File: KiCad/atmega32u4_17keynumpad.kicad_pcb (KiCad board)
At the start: 2 copper layers, 82 x 134 mm, 50 parts, among them SW1 1825115-1, SW10 MX1A-11NW, SW11 MX1A-11NW, SW118 MX1A-11NW, SW12 MX1A-11NW, SW13 MX1A-11NW, SW14 MX1A-11NW, SW15 MX1A-11NW, SW16 MX1A-11NW, SW17 MX1A-11NW, SW2 MX1A-11NW, SW3 MX1A-11NW, SW4 MX1A-11NW, SW5 MX1A-11NW, SW6 MX1A-11NW, SW7 MX1A-11NW, SW8 MX1A-11NW, SW9 MX1A-11NW

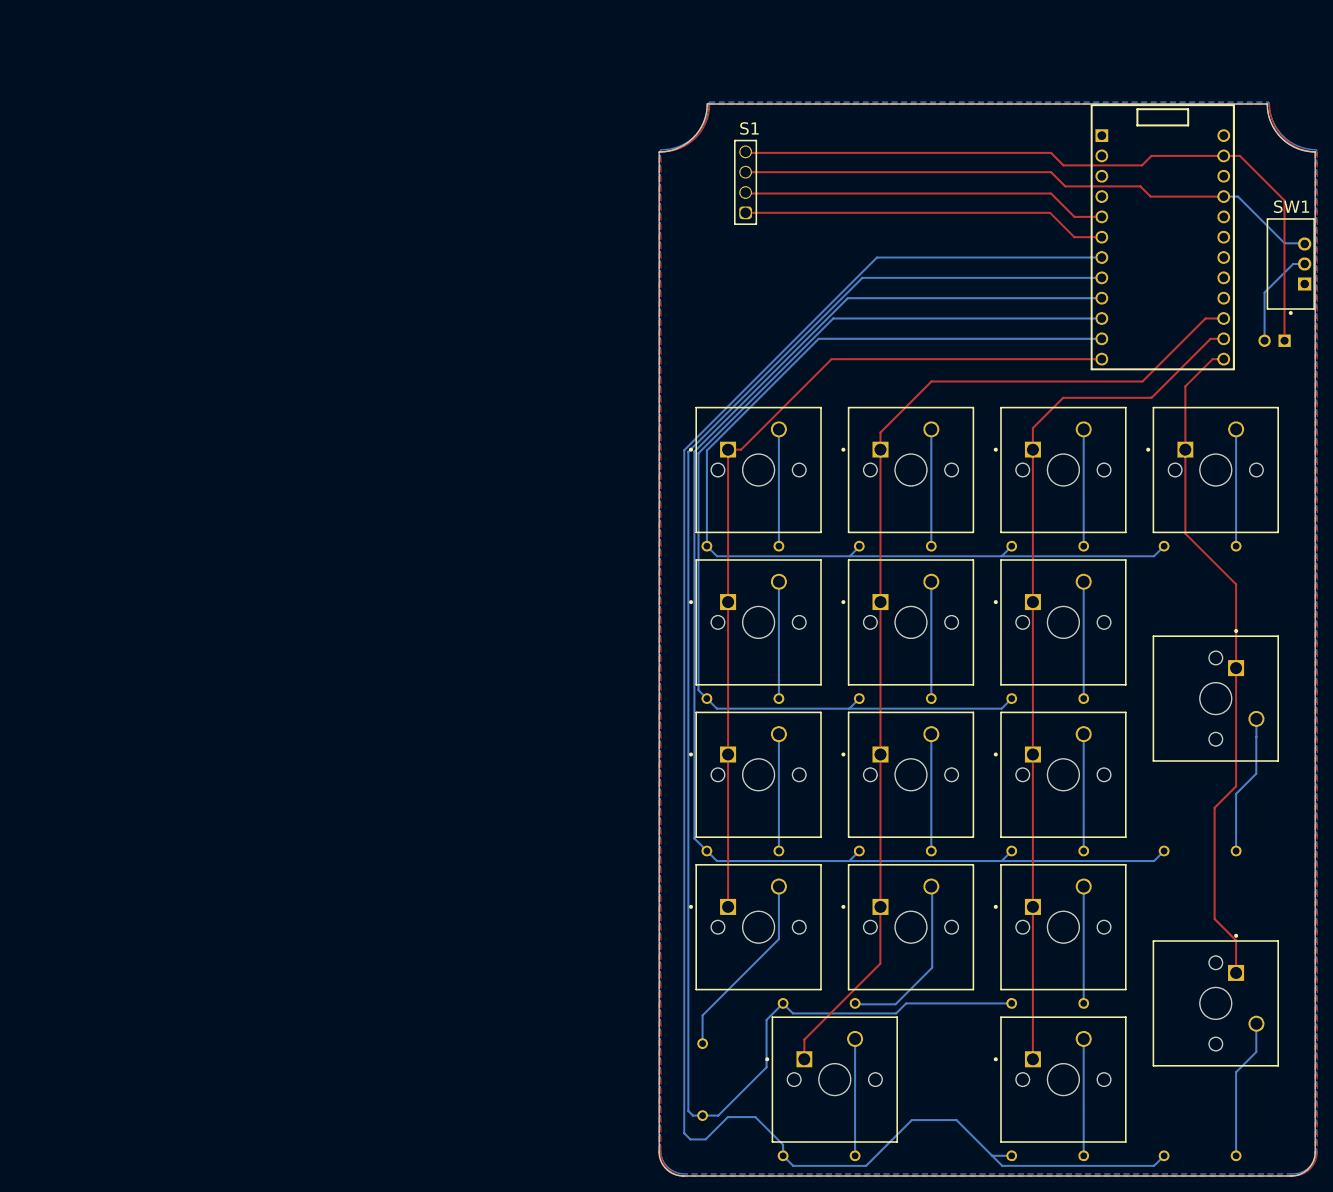
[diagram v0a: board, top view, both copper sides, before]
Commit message: finished pcb
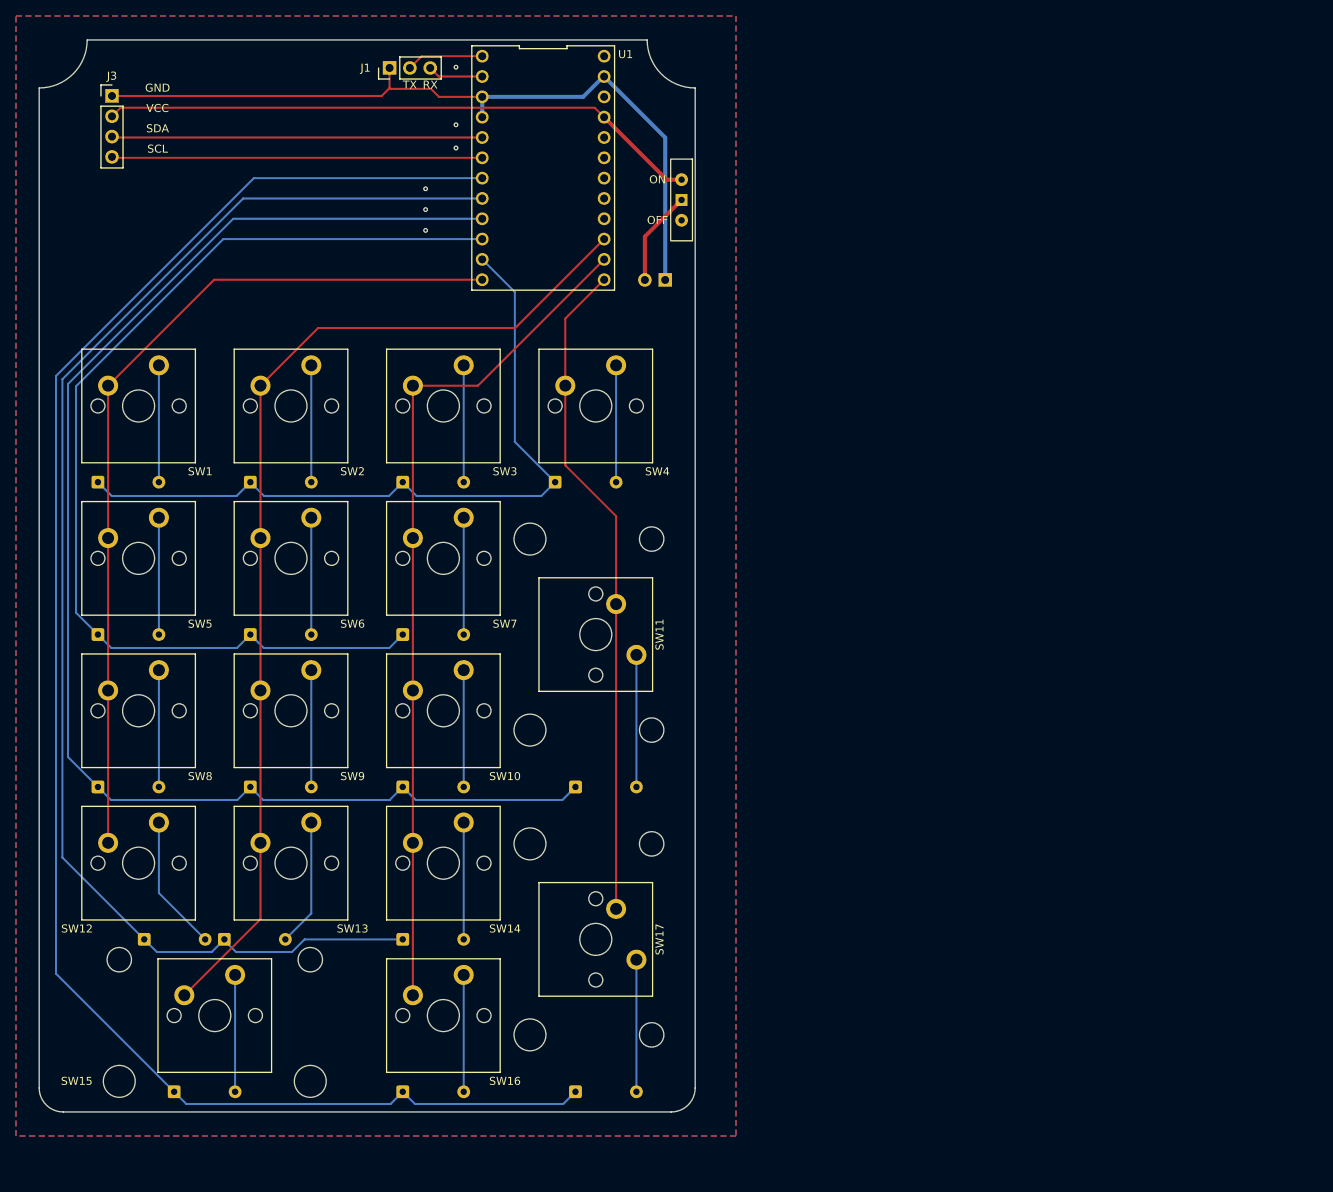
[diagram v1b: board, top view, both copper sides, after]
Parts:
- removed ? (x12): , 
- removed ?: PRO MICRO, PcbLib1:PRO MICRO
- removed B1: B2B-XH-A(LF)(SN), Vault:FP-B2B-XH-A_LF_SN-MFG
- removed D18: 1N4148, Vault:NXP-SOD27-2_V
- removed S1: 61300411121, Vault:61300411121
- removed SW118: MX1A-11NW, Vault:CHRY-MX1A-11NW_V
- added D1: 1N4148, Diode_THT:D_DO-35_SOD27_P7.62mm_Horizontal, B.Cu at (37.3, 85.3)
- added J1: Conn_01x03_Pin, Connector_PinHeader_2.54mm:PinHeader_1x03_P2.54mm_Vertical, F.Cu at (73.8, 33.5)
- added J2: power supply, Connector_PinSocket_2.54mm:PinSocket_1x02_P2.54mm_Vertical, B.Cu at (108.2, 60.0)
- added J3: LCD1602, Connector_PinHeader_2.54mm:PinHeader_1x04_P2.54mm_Vertical, F.Cu at (39.1, 37.0)
- added REF**: Stabilizer_Cherry_MX_2.00u, PCM_Mounting_Keyboard_Stabilizer:Stabilizer_Cherry_MX_2.00u, F.Cu at (99.6, 104.3)
- added REF**: Stabilizer_Cherry_MX_2.00u, PCM_Mounting_Keyboard_Stabilizer:Stabilizer_Cherry_MX_2.00u, F.Cu at (52.0, 151.9)
- added REF**: Stabilizer_Cherry_MX_2.00u, PCM_Mounting_Keyboard_Stabilizer:Stabilizer_Cherry_MX_2.00u, F.Cu at (99.6, 142.4)
- added SW18: slide_switch, Button_Switch_THT:SW_Slide-03_Wuerth-WS-SLTV_10x2.5x6.4_P2.54mm, F.Cu at (110.3, 50.0)
- added U1: Pro Micro, pro_micro:Pro Micro, F.Cu at (93.0, 46.0)
- D10, D11, D12, D13, D14, D15, D16, D17, D2, D3, D4, D5, D6, D7, D8, D9: footprint Vault:NXP-SOD27-2_V -> Diode_THT:D_DO-35_SOD27_P7.62mm_Horizontal
- SW1: value 1825115-1 -> SW_Push; footprint Vault:FP-1825115-1-MFG -> PCM_Switch_Keyboard_Cherry_MX:SW_Cherry_MX_PCB_1.00u
- SW10, SW12, SW13, SW14, SW16, SW2, SW3, SW4, SW5, SW6, SW7, SW8, SW9: value MX1A-11NW -> SW_Push; footprint Vault:CHRY-MX1A-11NW_V -> PCM_Switch_Keyboard_Cherry_MX:SW_Cherry_MX_PCB_1.00u
- SW11, SW15, SW17: value MX1A-11NW -> SW_Push; footprint Vault:CHRY-MX1A-11NW_V -> PCM_Switch_Keyboard_Cherry_MX:SW_Cherry_MX_PCB_2.00u
- moved SW1 145.1 mm to (42.4, 75.8), turned to 0 degrees
- moved D5 138.2 mm to (37.3, 104.3), turned to 0 degrees
- moved SW12 136.2 mm to (42.4, 132.9), turned to 0 degrees
- moved SW5 135.1 mm to (42.4, 94.8)
- moved D12 132.4 mm to (43.1, 142.4), turned to 0 degrees
- moved D8 119.2 mm to (37.3, 123.4), turned to 0 degrees
- moved SW8 116.1 mm to (42.4, 113.8)
- moved D15 109.8 mm to (46.9, 161.5), turned to 0 degrees
- moved SW15 106.6 mm to (52.0, 151.9)
- moved D13 62.3 mm to (53.1, 142.4), turned to 0 degrees
- moved D10 62.1 mm to (75.4, 123.4), turned to 0 degrees
- moved D3 62.1 mm to (75.4, 85.3), turned to 0 degrees
- moved D4 62.1 mm to (94.5, 85.3), turned to 0 degrees
- moved D7 62.1 mm to (75.4, 104.3), turned to 0 degrees
- moved D2 62.1 mm to (56.4, 85.3), turned to 0 degrees
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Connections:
- net NetMCU1_15 renamed /Pin 16 (COL 3)
- D10 pad 1: NetD10_1 -> /Pin 6 (ROW 3)
- D10 pad 2: NetD9_2 -> Net-(D10-A)
- D11 pad 1: NetD11_1 -> /Pin 6 (ROW 3)
- D11 pad 2: NetD9_2 -> Net-(D11-A)
- D12 pad 1: NetD12_1 -> /Pin 5 (ROW 4)
- D12 pad 2: NetD9_2 -> Net-(D12-A)
- D13 pad 1: NetD13_1 -> /Pin 5 (ROW 4)
- D13 pad 2: NetD13_2 -> Net-(D13-A)
- D14 pad 1: NetD14_1 -> /Pin 5 (ROW 4)
- D14 pad 2: NetD13_2 -> Net-(D14-A)
- D15 pad 1: NetD15_1 -> /Pin 4 (ROW 5)
- D15 pad 2: NetD13_2 -> Net-(D15-A)
- D16 pad 1: NetD16_1 -> /Pin 4 (ROW 5)
- D16 pad 2: NetD16_2 -> Net-(D16-A)
- D17 pad 1: NetD17_1 -> /Pin 4 (ROW 5)
- D17 pad 2: NetD16_2 -> Net-(D17-A)
- D2 pad 1: NetD2_1 -> /Pin 8 (ROW 1)
- D2 pad 2: NetD2_2 -> Net-(D2-A)
- D3 pad 1: NetD3_1 -> /Pin 8 (ROW 1)
- D3 pad 2: NetD2_2 -> Net-(D3-A)
- D4 pad 1: NetD4_1 -> /Pin 8 (ROW 1)
- D4 pad 2: NetD2_2 -> Net-(D4-A)
- D5 pad 1: NetD5_1 -> /Pin 7 (ROW 2)
- D5 pad 2: NetD2_2 -> Net-(D5-A)
- D6 pad 1: NetD6_1 -> /Pin 7 (ROW 2)
- D6 pad 2: NetD6_2 -> Net-(D6-A)
- D7 pad 1: NetD7_1 -> /Pin 7 (ROW 2)
- D7 pad 2: NetD6_2 -> Net-(D7-A)
- D8 pad 1: NetD8_1 -> /Pin 6 (ROW 3)
- D8 pad 2: NetD6_2 -> Net-(D8-A)
- D9 pad 1: NetD9_1 -> /Pin 6 (ROW 3)
- D9 pad 2: NetD9_2 -> Net-(D9-A)
- SW1 pad 1: (no net) -> /Pin 9 (COL 1)
- SW1 pad 2: NetJ1_2 -> Net-(D1-A)
- SW10 pad 2: NetD10_1 -> Net-(D10-A)
- SW11 pad 1: NetMCU1_14 -> /Pin 10 (COL 4)
- SW11 pad 2: NetD11_1 -> Net-(D11-A)
- SW12 pad 1: NetMCU1_13 -> /Pin 9 (COL 1)
- SW12 pad 2: NetD12_1 -> Net-(D12-A)
- SW13 pad 1: NetMCU1_12 -> /Pin 14 (COL 2)
- SW13 pad 2: NetD13_1 -> Net-(D13-A)
- SW14 pad 2: NetD14_1 -> Net-(D14-A)
- SW15 pad 1: NetMCU1_14 -> /Pin 14 (COL 2)
- SW15 pad 2: NetD15_1 -> Net-(D15-A)
- SW16 pad 2: NetD16_1 -> Net-(D16-A)
- SW17 pad 1: NetMCU1_14 -> /Pin 10 (COL 4)
- SW17 pad 2: NetD17_1 -> Net-(D17-A)
- SW2 pad 1: NetMCU1_12 -> /Pin 14 (COL 2)
- SW2 pad 2: NetD2_1 -> Net-(D2-A)
- SW3 pad 2: NetD3_1 -> Net-(D3-A)
- SW4 pad 1: NetMCU1_14 -> /Pin 10 (COL 4)
- SW4 pad 2: NetD4_1 -> Net-(D4-A)
- SW5 pad 1: NetMCU1_13 -> /Pin 9 (COL 1)
- SW5 pad 2: NetD5_1 -> Net-(D5-A)
- SW6 pad 1: NetMCU1_12 -> /Pin 14 (COL 2)
- SW6 pad 2: NetD6_1 -> Net-(D6-A)
- SW7 pad 2: NetD7_1 -> Net-(D7-A)
- SW8 pad 1: NetMCU1_14 -> /Pin 9 (COL 1)
- SW8 pad 2: NetD8_1 -> Net-(D8-A)
- SW9 pad 1: NetMCU1_12 -> /Pin 14 (COL 2)
- SW9 pad 2: NetD9_1 -> Net-(D9-A)
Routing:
- net NetD16_2: track 220.0 -> 0.00 mm
- net /Pin 4 (ROW 5): track 0.00 -> 212.0 mm
- net NetD13_2: track 194.1 -> 0.00 mm
- net /Pin 6 (ROW 3): track 0.00 -> 176.0 mm
- net NetD9_2: track 171.2 -> 0.00 mm
- net /Pin 5 (ROW 4): track 0.00 -> 171.1 mm
- net /Pin 7 (ROW 2): track 0.00 -> 131.4 mm
- net /Pin 14 (COL 2): track 0.00 -> 130.7 mm
- net NetD6_2: track 129.4 -> 0.00 mm
- net NetD2_2: track 129.0 -> 0.00 mm
- net /Pin 9 (COL 1): track 0.00 -> 109.4 mm
- net NetMCU1_12: track 108.6 -> 0.00 mm
- net NetMCU1_14: track 107.4 -> 0.00 mm
- net /Pin 8 (ROW 1): track 0.00 -> 93.1 mm
- net NetMCU1_13: track 84.4 -> 0.00 mm
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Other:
- board text added: "GND"
- board text added: "OFF"
- board text added: "ON"
- board text added: "RX"
- board text added: "SCL"
- board text added: "SDA"
- board text added: "TX"
- board text added: "VCC"
- board text removed: "Techniki Analogowe czy cos"
